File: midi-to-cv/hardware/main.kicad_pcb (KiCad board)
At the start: 2 copper layers, 63.5 x 51.6 mm, 19 parts, among them J1 audio-jack, J2 DIN_5, J3 SERIAL, J4 ICSP, J5 5V, U1 6N137, U2 MCP4921-E/P, U3 ATTINY2313-P, Y1 16MHz

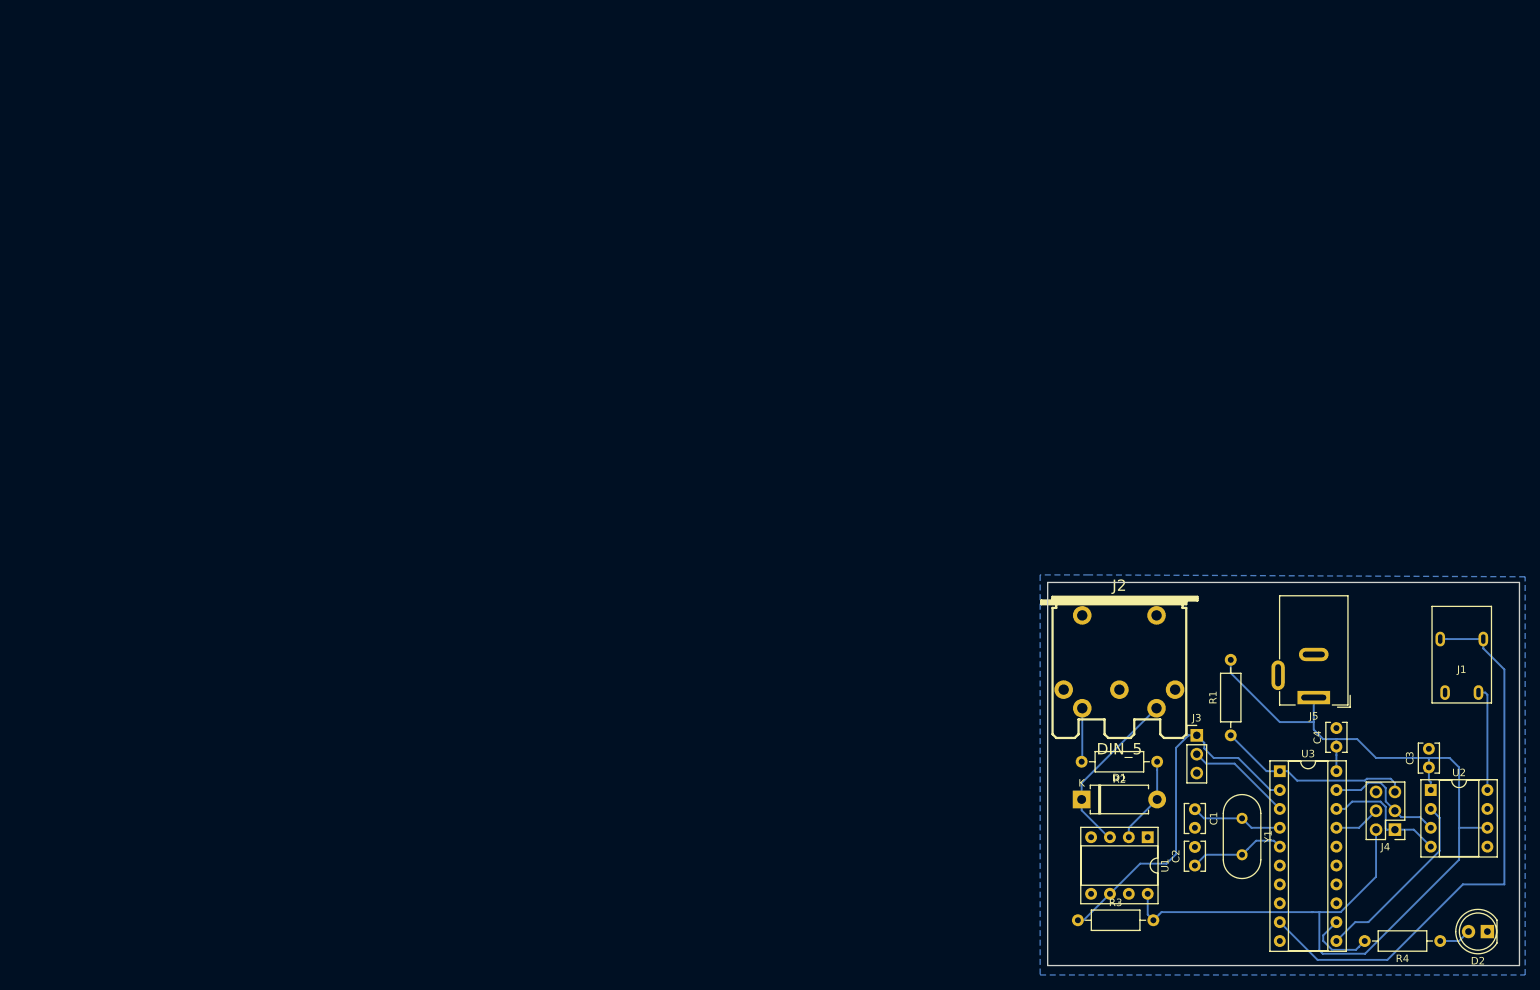
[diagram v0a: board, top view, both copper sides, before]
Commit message: midi-to-cv: revision 3
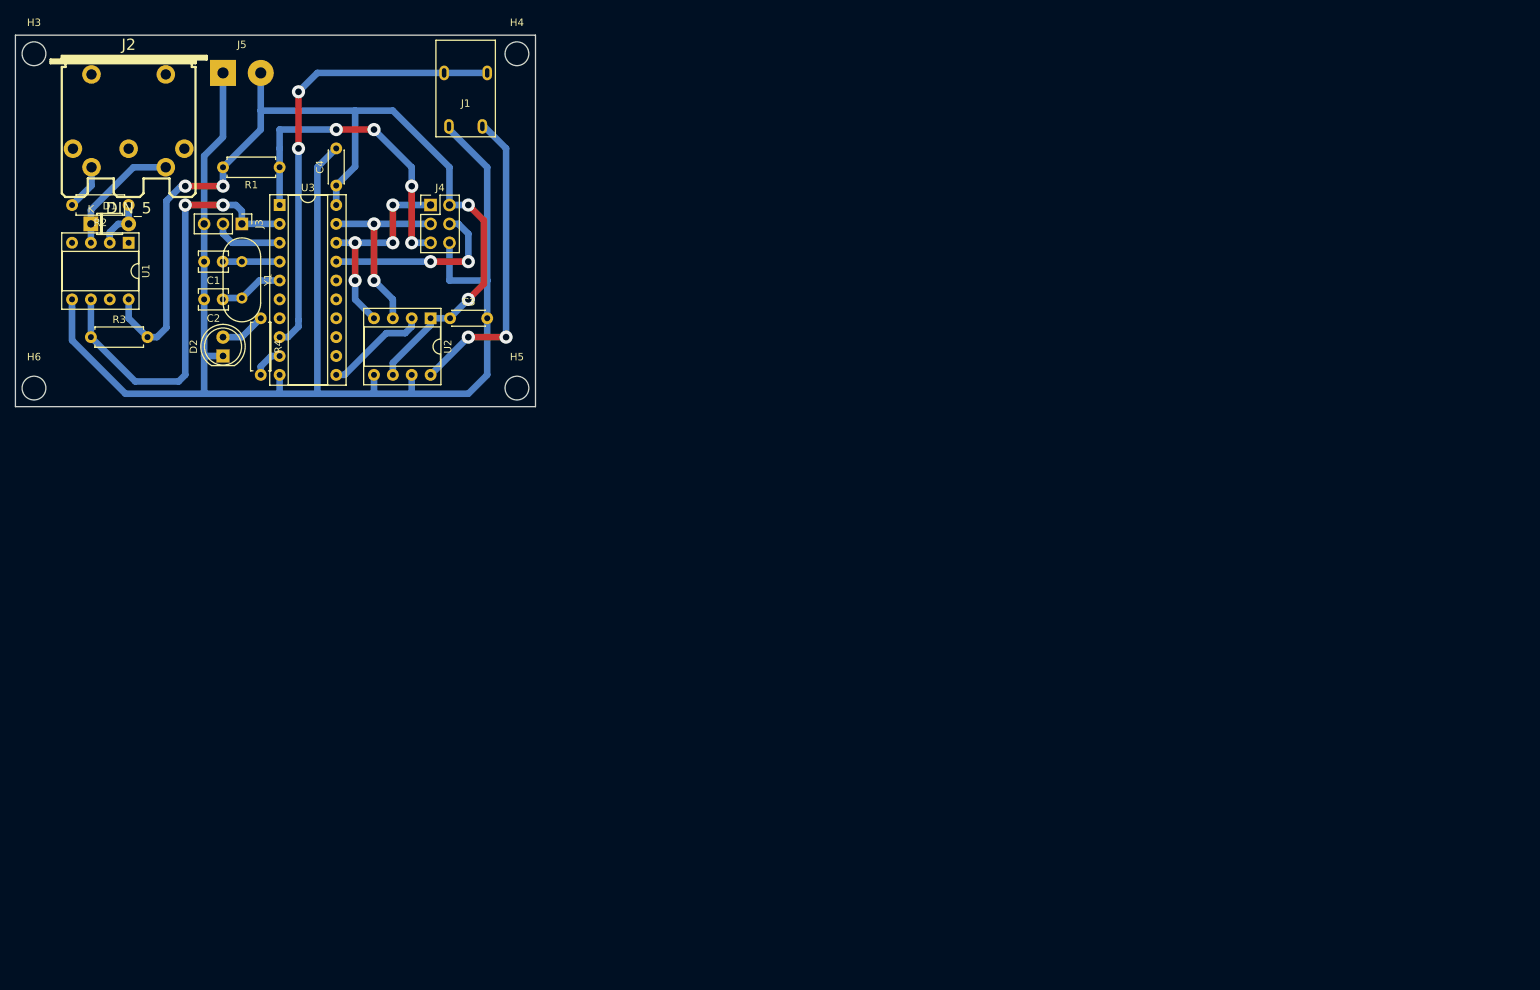
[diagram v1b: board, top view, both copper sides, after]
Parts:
- added H3: MountingHole, MountingHole:MountingHole_3.2mm_M3, F.Cu at (2.50, 2.50)
- added H4: MountingHole, MountingHole:MountingHole_3.2mm_M3, F.Cu at (67.5, 2.50)
- added H5: MountingHole, MountingHole:MountingHole_3.2mm_M3, F.Cu at (67.5, 47.5)
- added H6: MountingHole, MountingHole:MountingHole_3.2mm_M3, F.Cu at (2.50, 47.5)
- C3, C4: footprint Capacitor_THT:C_Disc_D3.8mm_W2.6mm_P2.50mm -> Capacitor_THT:C_Disc_D4.3mm_W1.9mm_P5.00mm
- D1: footprint Diode_THT:D_DO-15_P10.16mm_Horizontal -> Diode_THT:D_T-1_P5.08mm_Horizontal
- J5: value 5V -> Conn_01x02_Male; footprint Connector_BarrelJack:BarrelJack_Wuerth_6941xx301002 -> Connector_Wire:SolderWirePad_1x02_P5.08mm_Drill1.5mm
- R1, R2, R3, R4: footprint Resistor_THT:R_Axial_DIN0207_L6.3mm_D2.5mm_P10.16mm_Horizontal -> Resistor_THT:R_Axial_DIN0207_L6.3mm_D2.5mm_P7.62mm_Horizontal
- moved D2 187.0 mm to (27.9, 43.2), turned to 90 degrees
- moved R4 179.5 mm to (33.0, 38.1), turned to 270 degrees
- moved J5 169.2 mm to (27.9, 5.08), turned to 0 degrees
- moved U1 158.8 mm to (15.2, 27.9)
- moved R2 157.4 mm to (15.2, 22.9)
- moved U3 154.7 mm to (35.6, 22.9)
- moved J4 154.6 mm to (55.9, 22.9), turned to 0 degrees
- moved C4 154.4 mm to (43.2, 20.2)
- moved R3 154.3 mm to (10.2, 40.6)
- moved D1 154.2 mm to (10.2, 25.4)
- moved J1 154.2 mm to (60.6, 8.68)
- moved Y1 154.1 mm to (30.5, 30.5)
- moved J2 151.9 mm to (15.2, 12.3)
- moved C2 151.4 mm to (27.9, 35.6), turned to 180 degrees
- moved C1 150.2 mm to (27.9, 30.5), turned to 180 degrees
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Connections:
- J5 pad 1: VCC -> GND
- J5 pad 2: GND -> VCC
- U3 pad 12: Net-(R4-Pad2) -> Net-(U3-Pad12)
- U3 pad 8: Net-(U3-Pad8) -> TRIG
- U3 pad 9: TRIG -> Net-(R4-Pad2)
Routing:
- net GND: track 0.00 -> 199.6 mm
- net DACOUT: track 14.2 -> 42.1 mm, vias 0 -> 2
- net MOSI: track 6.28 -> 24.6 mm, vias 0 -> 2
- net RST: track 26.2 -> 42.7 mm, vias 0 -> 4
- net TRIG: track 76.5 -> 61.2 mm, vias 0 -> 2
- net DO: track 17.3 -> 29.0 mm, vias 0 -> 4
- net ~CS: track 25.1 -> 14.0 mm
- net SCK: track 16.7 -> 26.5 mm, vias 0 -> 2
- net RX: track 49.4 -> 58.3 mm, vias 0 -> 2
- net VCC: track 140.1 -> 132.3 mm, vias 0 -> 4
- net Net-(D1-Pad1): track 23.2 -> 16.9 mm
- net Net-(R4-Pad2): track 9.84 -> 4.25 mm
- net Net-(C1-Pad1): track 12.5 -> 7.66 mm
- net Net-(D1-Pad2): track 11.7 -> 6.96 mm
- net TX: track 14.2 -> 9.45 mm
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- removed copper zone on B.Cu, net GND
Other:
- board size 63.5 x 51.6 mm -> 70 x 50 mm
- net class Default: clearance 0.26 -> 0.635; trace_width 0.26 -> 0.889; via_dia 1 -> 1.778; via_drill 0.5 -> 0.889
- rule trace_clearance: 0.26 -> 0.635
- rule trace_min: 0.25 -> 0.889
- rule via_min_drill: 0.35 -> 0.889
- rule via_min_size: 0.5 -> 1.778
